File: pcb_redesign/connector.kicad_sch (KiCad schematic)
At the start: 8 parts, among them J1 USB_B_Mini, U3 SPX1117M3-L-3-3/TR

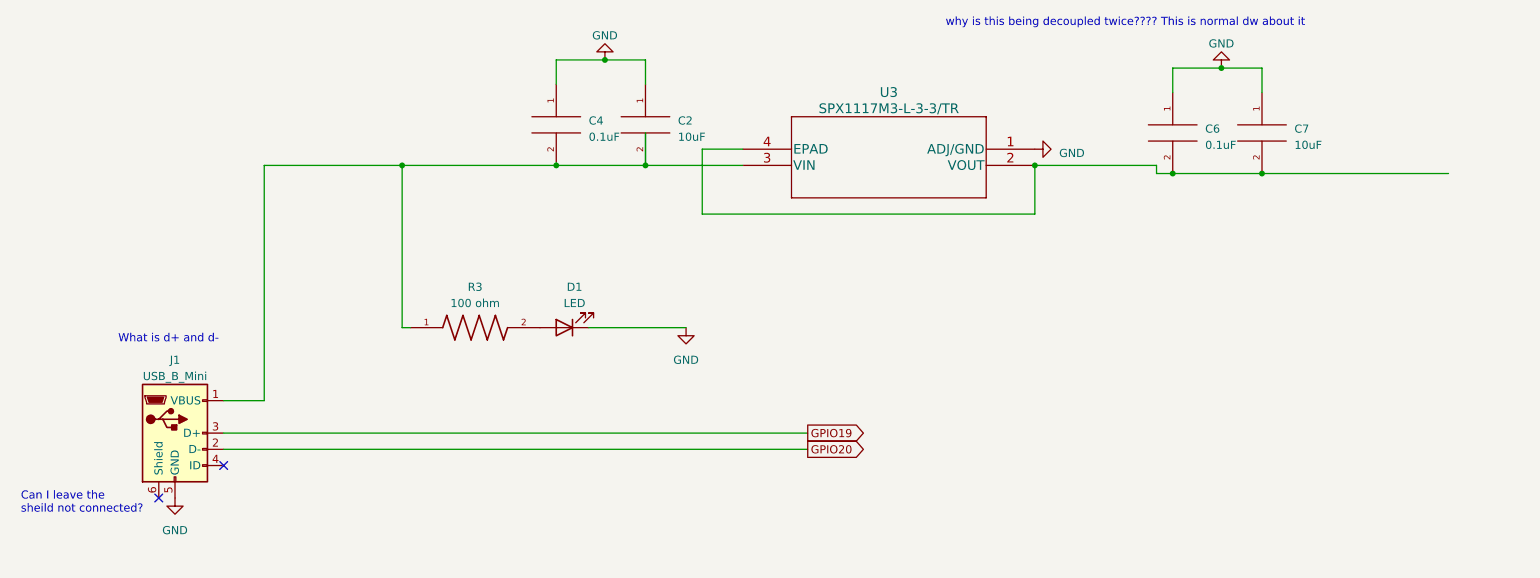
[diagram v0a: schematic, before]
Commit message: components added to board
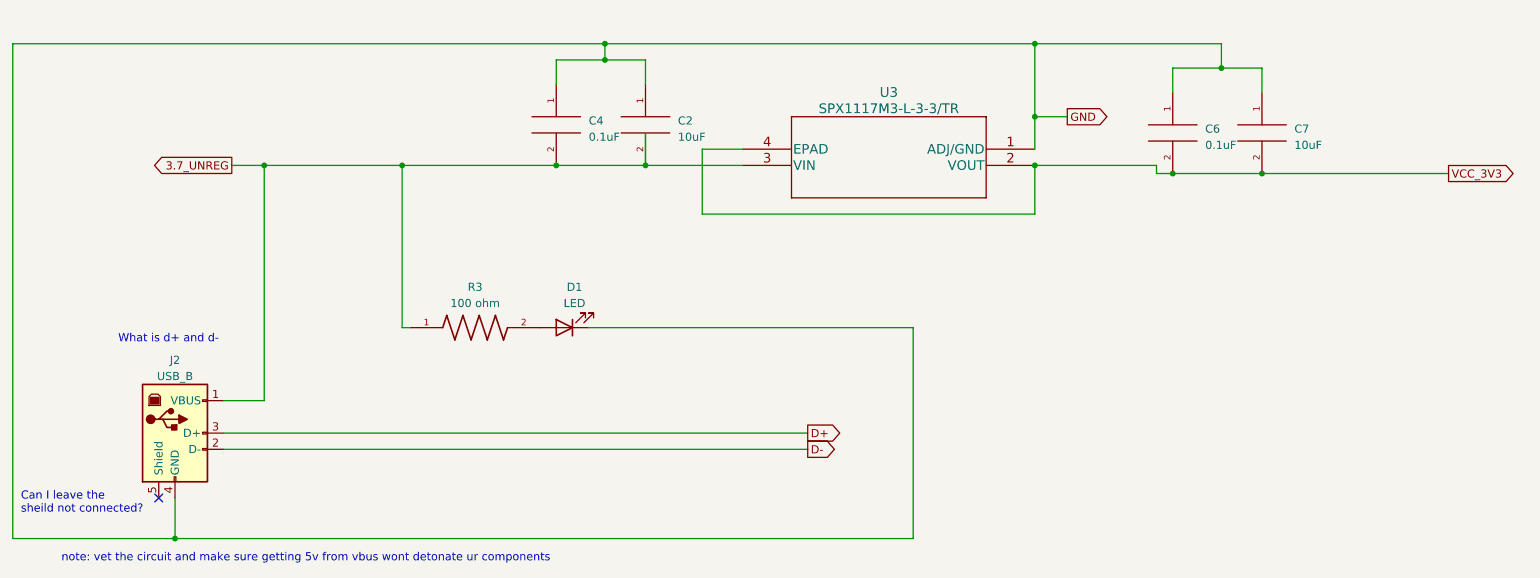
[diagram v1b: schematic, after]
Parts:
- removed J1: USB_B_Mini, micro_usb_type_b:AMPHENOL_10118192-0002LF, symbol Connector:USB_B_Mini
- added J2: USB_B, micro_usb_type_b:AMPHENOL_10118192-0002LF, symbol Connector:USB_B
- D1: footprint green_LED:LEDC2012X70N -> LED_SMD:LED_0805_2012Metric
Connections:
- net GND: now also J2.4 (GND)
- net 3.7_UNREG: now reaches C2.2, C4.2, R3.1, U3.3 (VIN)
- net 3.7_UNREG: now also J2.1 (VBUS)
- net VCC_3V3: now reaches C6.2, C7.2, U3.2 (VOUT), U3.4 (EPAD)
- new net D+: J2.3 (D+)
- new net D-: J2.2 (D-)
- no-connect marks 2 -> 1
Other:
- note added: "note: vet the circuit and make sure getting 5v from vbus wont detonate ur components"
- note removed: "why is this being decoupled twice???? This is normal dw about it"
